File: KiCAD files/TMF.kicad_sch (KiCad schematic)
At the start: 11 parts, among them J1 Conn_01x04_Pin, J2 Conn_01x04_Pin

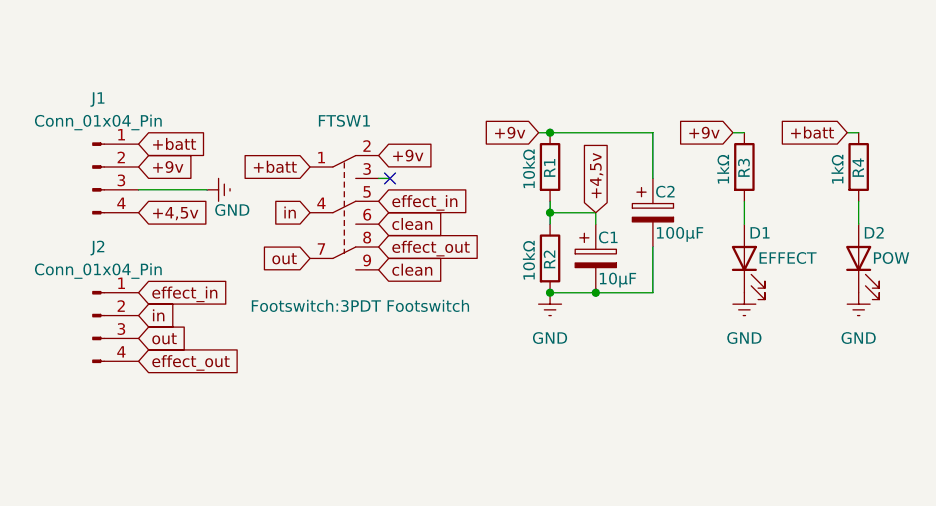
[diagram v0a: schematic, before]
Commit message: Redone PCB
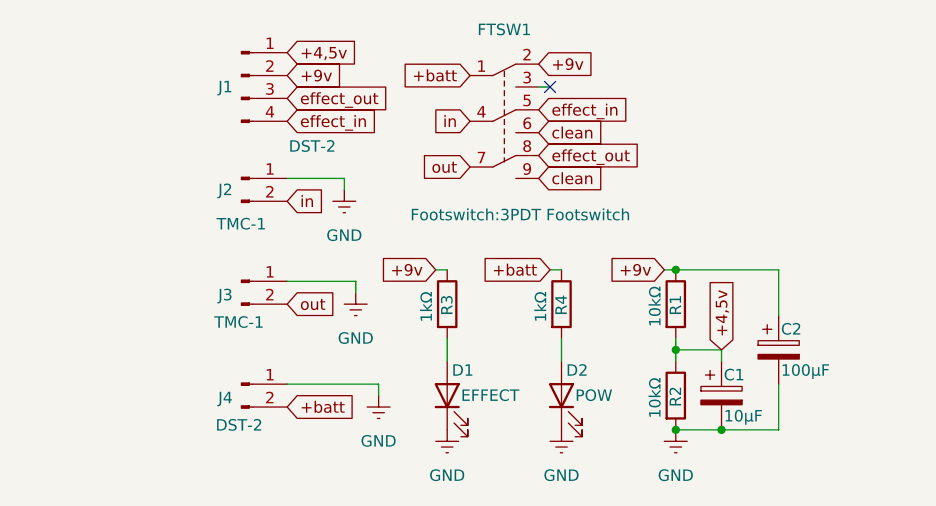
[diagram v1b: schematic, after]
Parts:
- removed J2: Conn_01x04_Pin, Connector_Hirose:Hirose_DF13-04P-1.25DSA_1x04_P1.25mm_Vertical, symbol Connector:Conn_01x04_Pin
- added J2, J3: TMC-1, Connector_JST:JST_XH_B2B-XH-A_1x02_P2.50mm_Vertical, symbol Connector:Conn_01x02_Pin
- added J4: DST-2, Connector_JST:JST_XH_B2B-XH-A_1x02_P2.50mm_Vertical, symbol Connector:Conn_01x02_Pin
- J1: value Conn_01x04_Pin -> DST-2; footprint Connector_Hirose:Hirose_DF13-04P-1.25DSA_1x04_P1.25mm_Vertical -> Connector_JST:JST_XH_B4B-XH-A_1x04_P2.50mm_Vertical
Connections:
- net +4,5v: now also J1.1 (Pin_1); no longer J1.4 (Pin_4)
- net +batt: now also J4.2 (Pin_2); no longer J1.1 (Pin_1)
- net GND: now also J2.1 (Pin_1), J3.1 (Pin_1), J4.1 (Pin_1); no longer J1.3 (Pin_3)
- net effect_in: now also J1.4 (Pin_4)
- net effect_out: now also J1.3 (Pin_3)
- net in: now also J2.2 (Pin_2)
- net out: now also J3.2 (Pin_2)
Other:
- moved on the sheet: C1, C2, D1, D2, FTSW1, J1, R1, R2, R3, R4
